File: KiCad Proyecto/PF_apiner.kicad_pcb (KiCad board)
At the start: 2 copper layers, 50 x 40.5 mm, 136 parts, among them J1 OBDII Header, J2 Conn_01x05, Q1 2N7002, Q10 2N7002, Q2 BSS314PE, Q3 BSS314PE, Q4 MMBT3904, Q5 MMBT3904, Q6 2N7002, Q7 2N7002, Q8 2N7002, Q9 BSS314PE, SW1 SW_RESET, SW2 SW_BOOT, U1 TPS54202, U10 STN2120, U11 AZ1117EH-3.3TRG1, U14 ESP32-WROOM, U2 AZ1117EH-3.3TRG1, U3 LM339, U4 MCP25612FD, U5 TH8056, U6 PESD1CAN, U7 PESD1CAN, U8 PESD1CAN, U9 LM317, Y1 16M

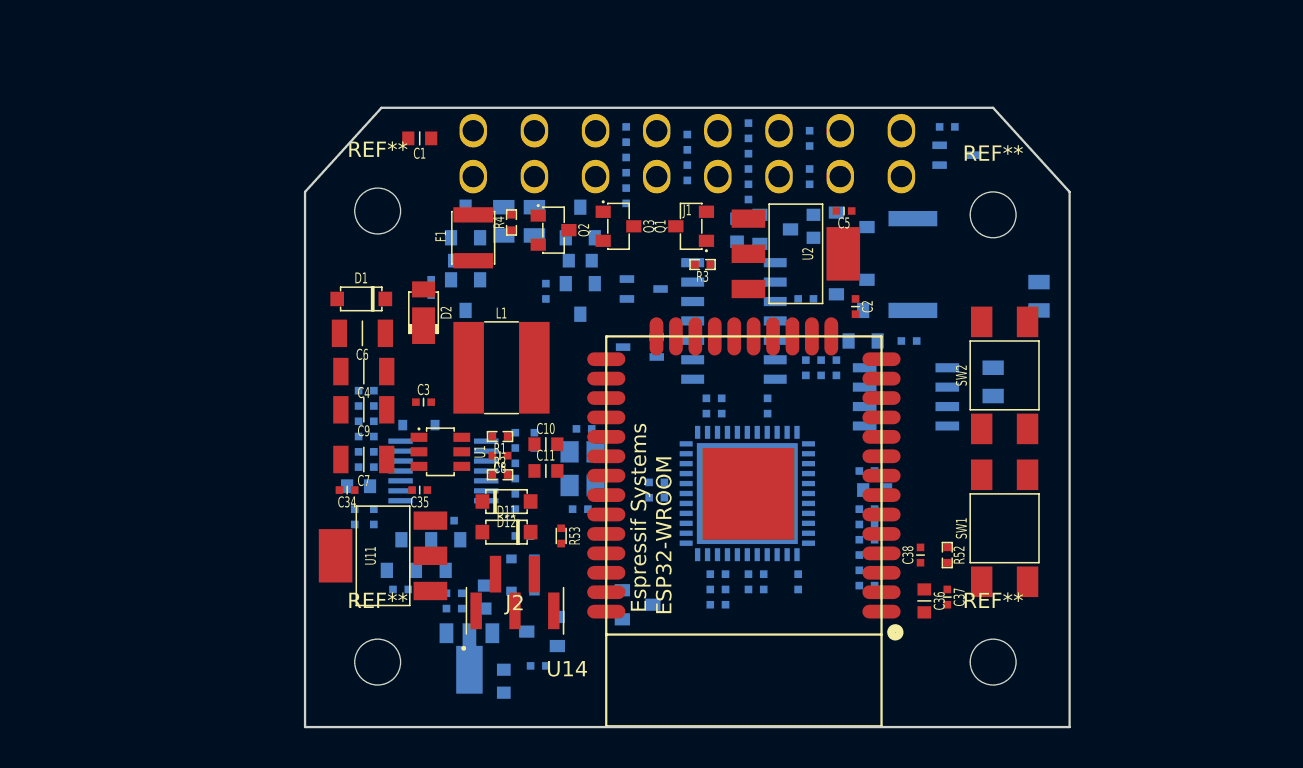
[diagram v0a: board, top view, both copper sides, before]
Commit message: modificado pcb
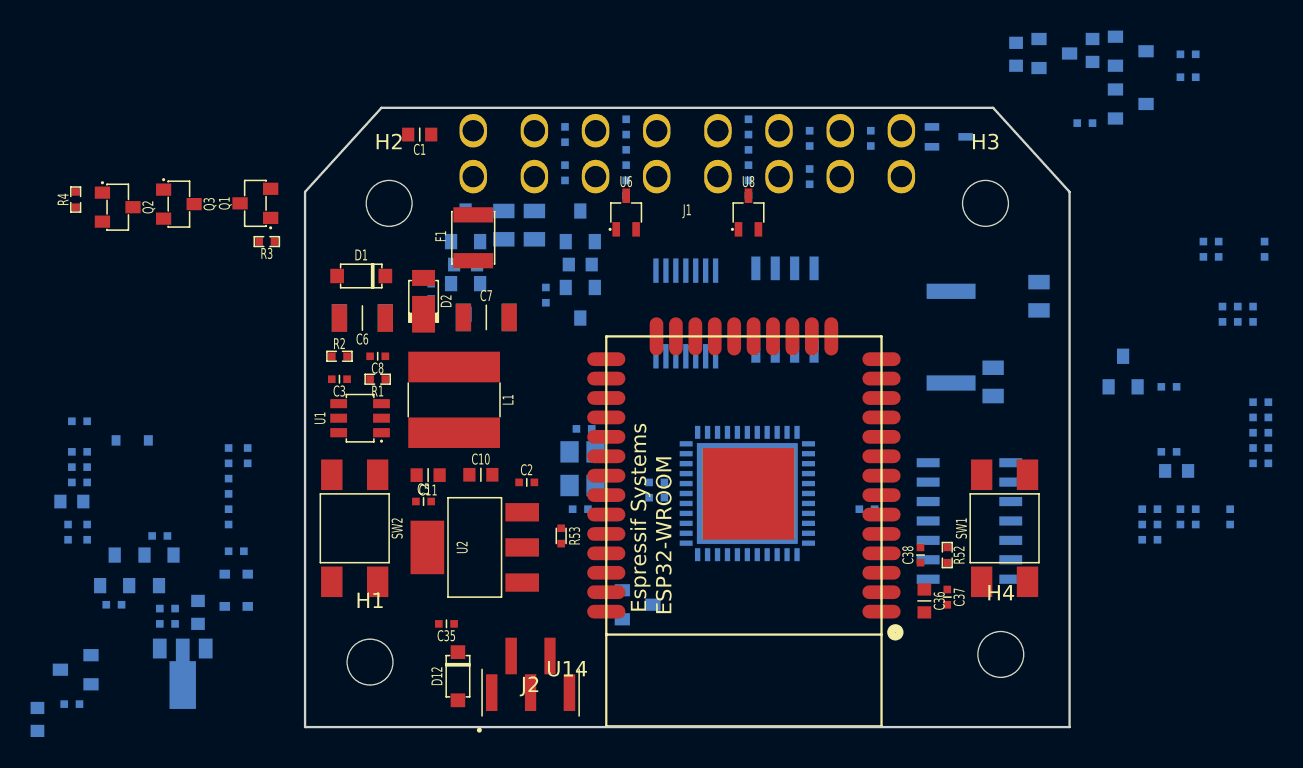
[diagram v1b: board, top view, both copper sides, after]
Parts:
- removed C34: 1uF, chip_rlc:c_0402
- removed D11: MBR0520, to-sod-sot:SOD-123
- removed REF** (x4): MountingHole_3mm, misc:MountingHole_3mm
- removed U11: AZ1117EH-3.3TRG1, to-sod-sot:SOT-223
- added H1: PCB_HOLE, misc:MountingHole_3mm, F.Cu at (84.2, 73.2)
- added H2: PCB_HOLE, misc:MountingHole_3mm, F.Cu at (85.5, 43.2)
- added H3: PCB_HOLE, misc:MountingHole_3mm, F.Cu at (124.5, 43.2)
- added H4: PCB_HOLE, misc:MountingHole_3mm, F.Cu at (125.5, 72.8)
- C4, C9: moved to B.Cu
- U6, U8: moved to F.Cu
- moved R31 58.9 mm to (137.8, 33.5)
- moved R38 57.5 mm to (137.8, 35.0)
- moved SW2 43.7 mm to (83.2, 64.5), turned to 270 degrees
- moved R49 34.1 mm to (138.8, 46.2)
- moved R50 34.1 mm to (139.8, 46.2)
- moved R51 34.1 mm to (142.8, 46.2)
- moved C5 33.4 mm to (87.8, 62.8), turned to 0 degrees
- moved C27 30.6 mm to (62.5, 77.0)
- moved Q7 30.6 mm to (65.0, 73.8)
- moved R27 30.6 mm to (64.8, 76.0)
- moved Q3 28.8 mm to (71.8, 43.3)
- moved C12 28.6 mm to (135.2, 65.2)
- moved C28 28.6 mm to (138.2, 63.8)
- moved R45 28.6 mm to (137.2, 63.8)
- moved R46 28.6 mm to (140.5, 63.8)
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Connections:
- net /HS_CAN_N renamed /CAN_Transceiver/HS_CAN_LO
- net /HS_CAN_P renamed /CAN_Transceiver/HS_CAN_HI
- net /J1850_BUS+ renamed /J1850_Transceiver/J1850_BUS+
- net /J1850_BUS- renamed /J1850_Transceiver/J1850_BUS-
- net /K-LINE renamed /ISO_Transceiver/K-LINE
- net /L-LINE renamed /ISO_Transceiver/L-LINE
- net /MS_CAN_N renamed /CAN_Transceiver/MS_CAN_LO
- net /MS_CAN_P renamed /CAN_Transceiver/MS_CAN_HI
- net /SW_CAN renamed /CAN_Transceiver/SW_CAN
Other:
- copper layers 2 -> 4
- net class Default: trace_width 0.1524 -> 0.15; via_dia 0.6096 -> 0.6; via_drill 0.4064 -> 0.4
- rule trace_min: 0.1524 -> 0.15
- rule via_min_drill: 0.4064 -> 0.4
- rule via_min_size: 0.6096 -> 0.6
